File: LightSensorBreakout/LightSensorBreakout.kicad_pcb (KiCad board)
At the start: 2 copper layers, 22 x 4 mm, 6 parts, among them U1 OPT4003DNPRQ1

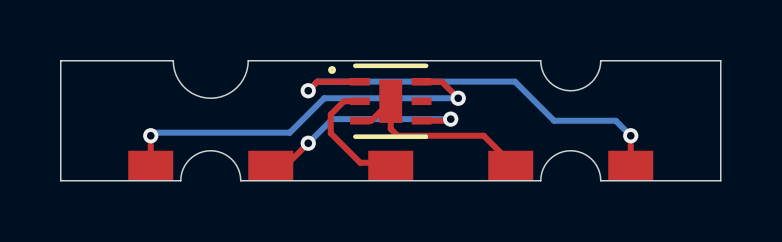
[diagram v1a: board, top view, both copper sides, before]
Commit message: V4 Updates
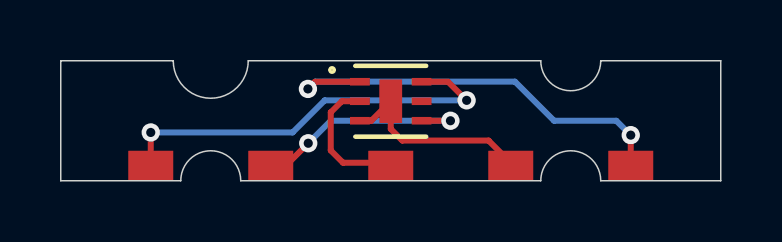
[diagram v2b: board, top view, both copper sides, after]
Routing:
- net /SDA: track 13.1 -> 13.7 mm
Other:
- board text added: "ARGUS CUBESAT"
